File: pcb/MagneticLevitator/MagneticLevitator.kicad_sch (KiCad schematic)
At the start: 14 parts, among them J1 ESP32 Left Side Pins, J2 ESP32 Right Side Pins, J3 Screw_Terminal_01x02, J4 Screw_Terminal_01x02, J6 hall effect sensor breakout, Q1 Q_NMOS_GDS, U1 LM7805_TO220

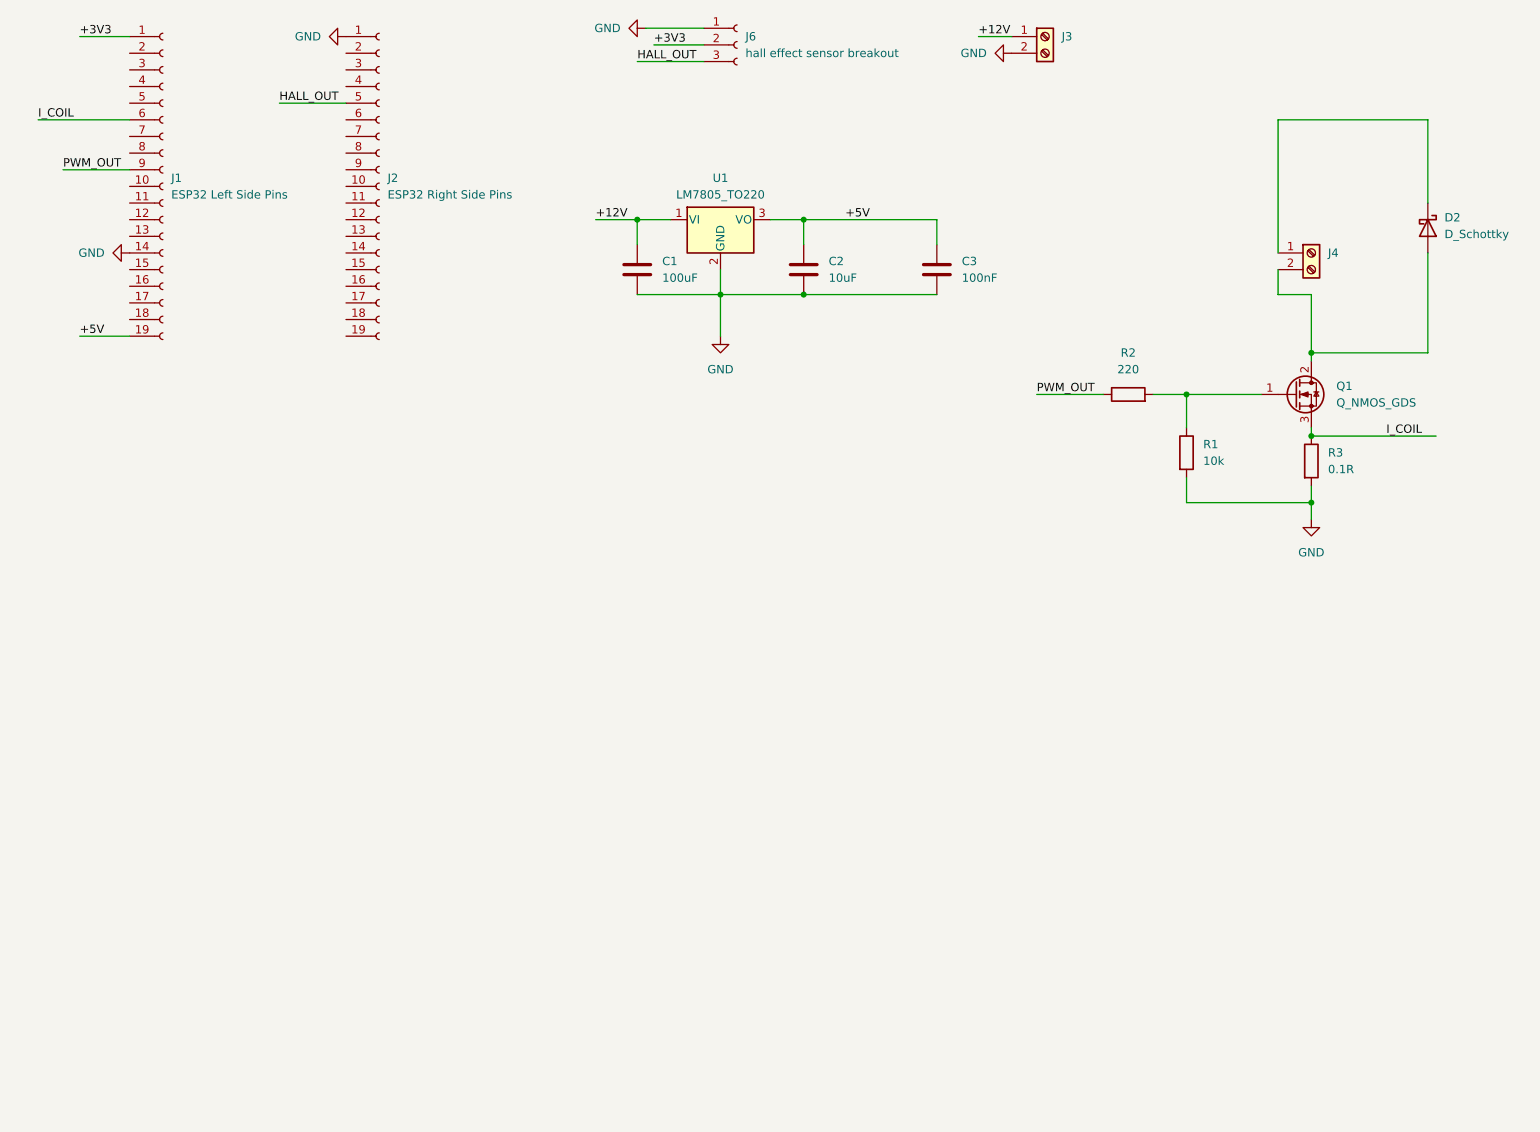
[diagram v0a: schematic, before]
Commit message: more PCB updates
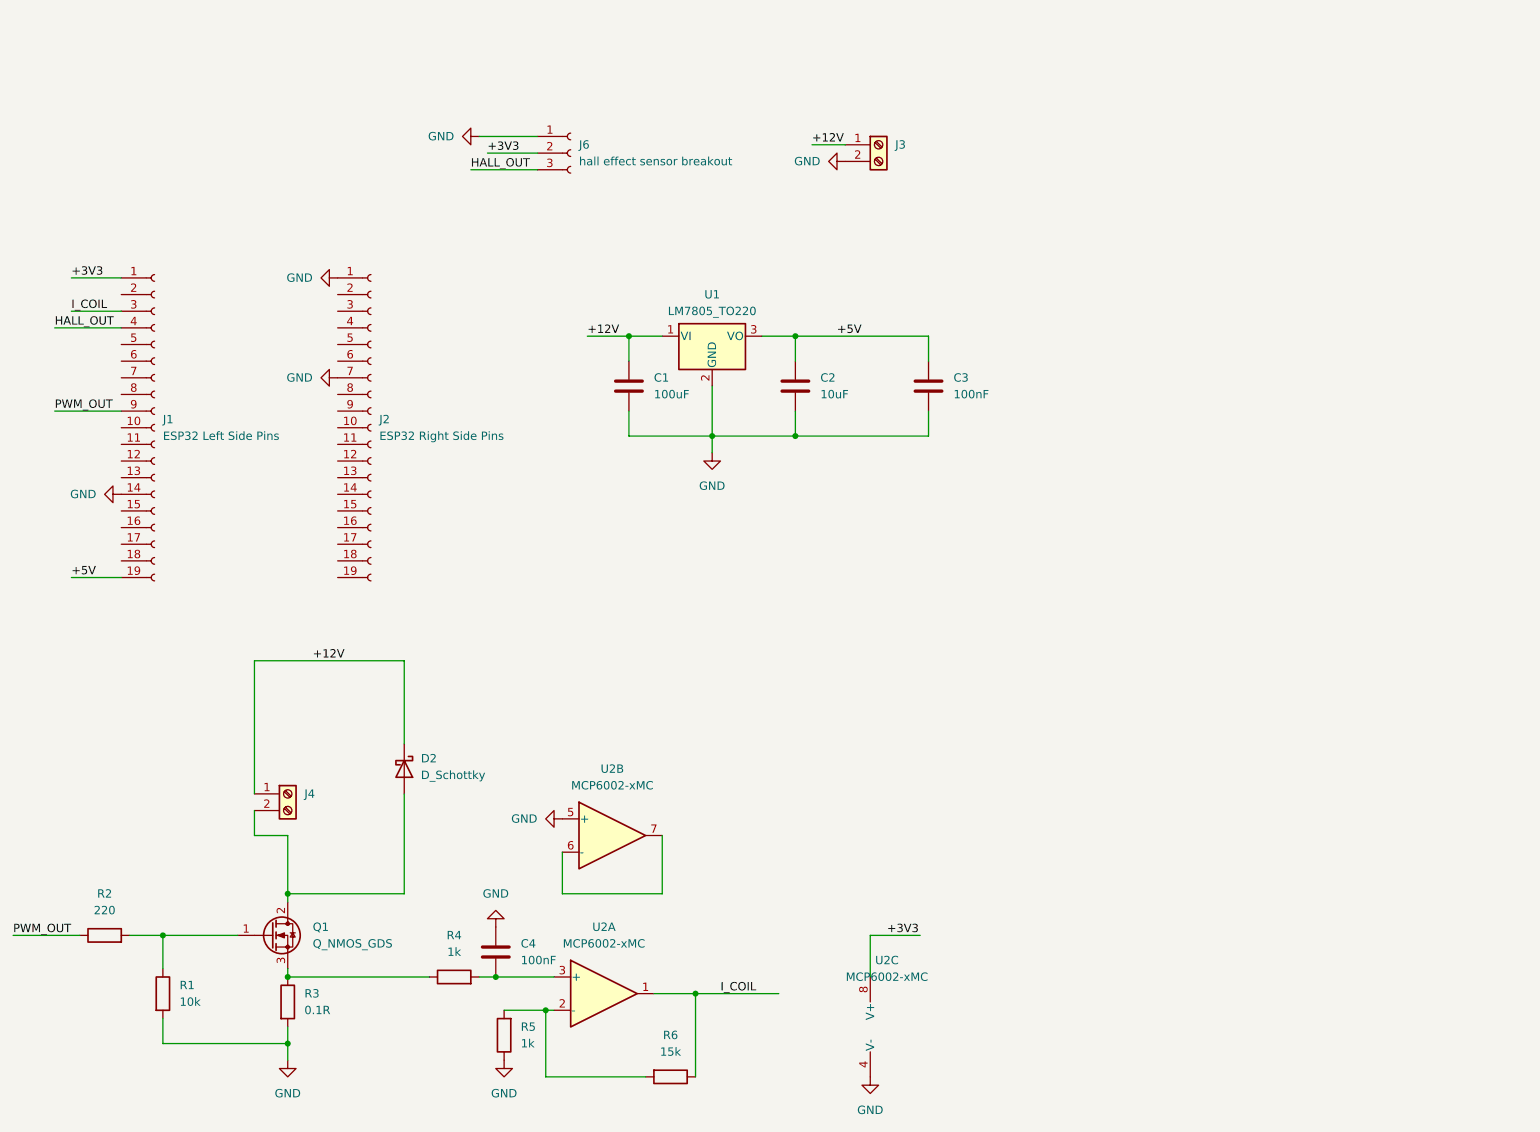
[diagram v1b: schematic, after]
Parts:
- added C4: 100nF, Capacitor_THT:C_Disc_D3.0mm_W1.6mm_P2.50mm, symbol Device:C
- added R4, R5: 1k, Resistor_THT:R_Axial_DIN0207_L6.3mm_D2.5mm_P10.16mm_Horizontal, symbol Device:R
- added R6: 15k, Resistor_THT:R_Axial_DIN0207_L6.3mm_D2.5mm_P10.16mm_Horizontal, symbol Device:R
- added U2: MCP6002-xMC, Package_DIP:DIP-8_W7.62mm, symbol Amplifier_Operational:MCP6002-xMC
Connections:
- net +12V: now also D2.1 (K), J4.1 (Pin_1)
- net +3V3: now also U2.8 (V+)
- net GND: now also J2.7 (Pin_7), C4.1, R5.1, U2.4 (V-), U2.5 (+), U2.9 (V-)
- net HALL_OUT: now also J1.4 (Pin_4); no longer J2.5 (Pin_5)
- net I_COIL: now also J1.3 (Pin_3), R6.1, U2.1; no longer J1.6 (Pin_6), Q1.3 (S), R3.1
- new net: R5.2, R6.2, U2.2 (-)
- new net: C4.2, R4.2, U2.3 (+)
- new net: U2.6 (-), U2.7
- new net: Q1.3 (S), R3.1, R4.1
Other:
- moved on the sheet: C1, C2, C3, D2, J1, J2, J3, J4, J6, Q1, R1, R2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
